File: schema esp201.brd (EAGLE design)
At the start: 100 x 80 mm, 9 parts

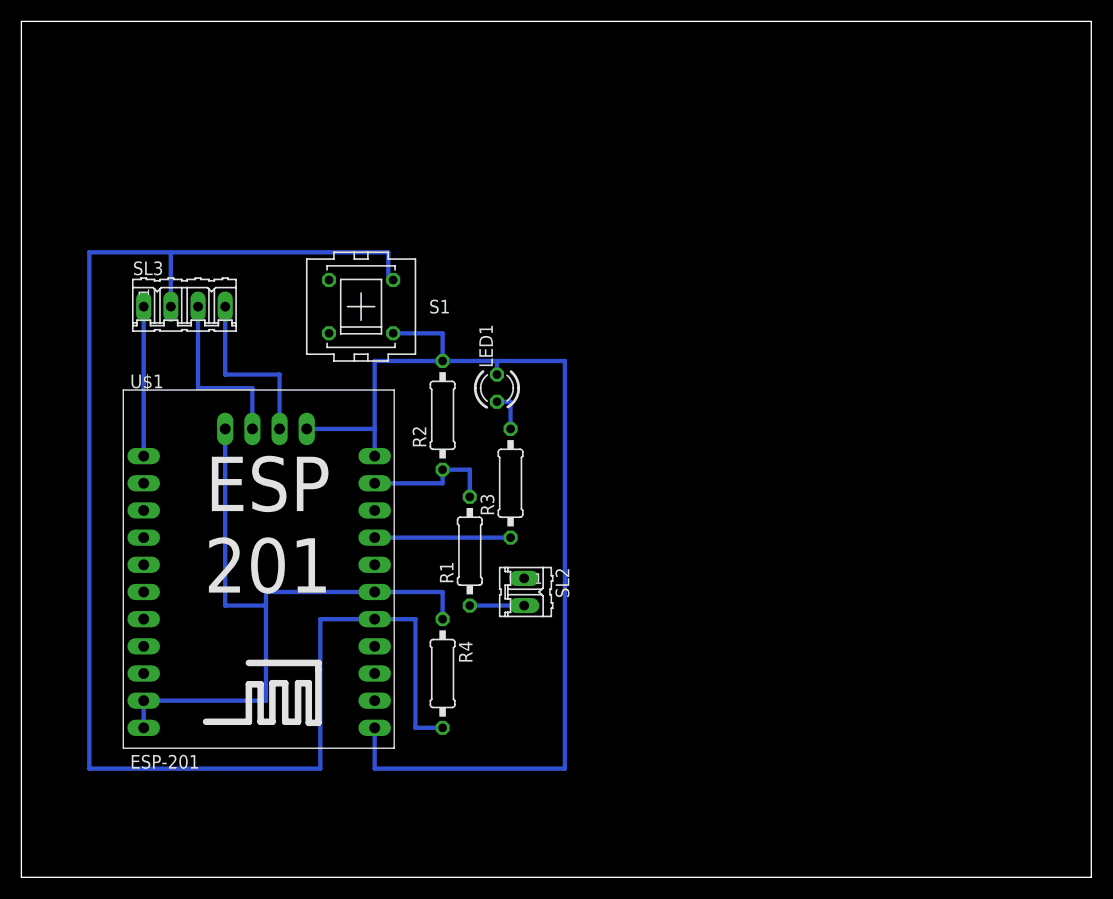
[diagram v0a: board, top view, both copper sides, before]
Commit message: +
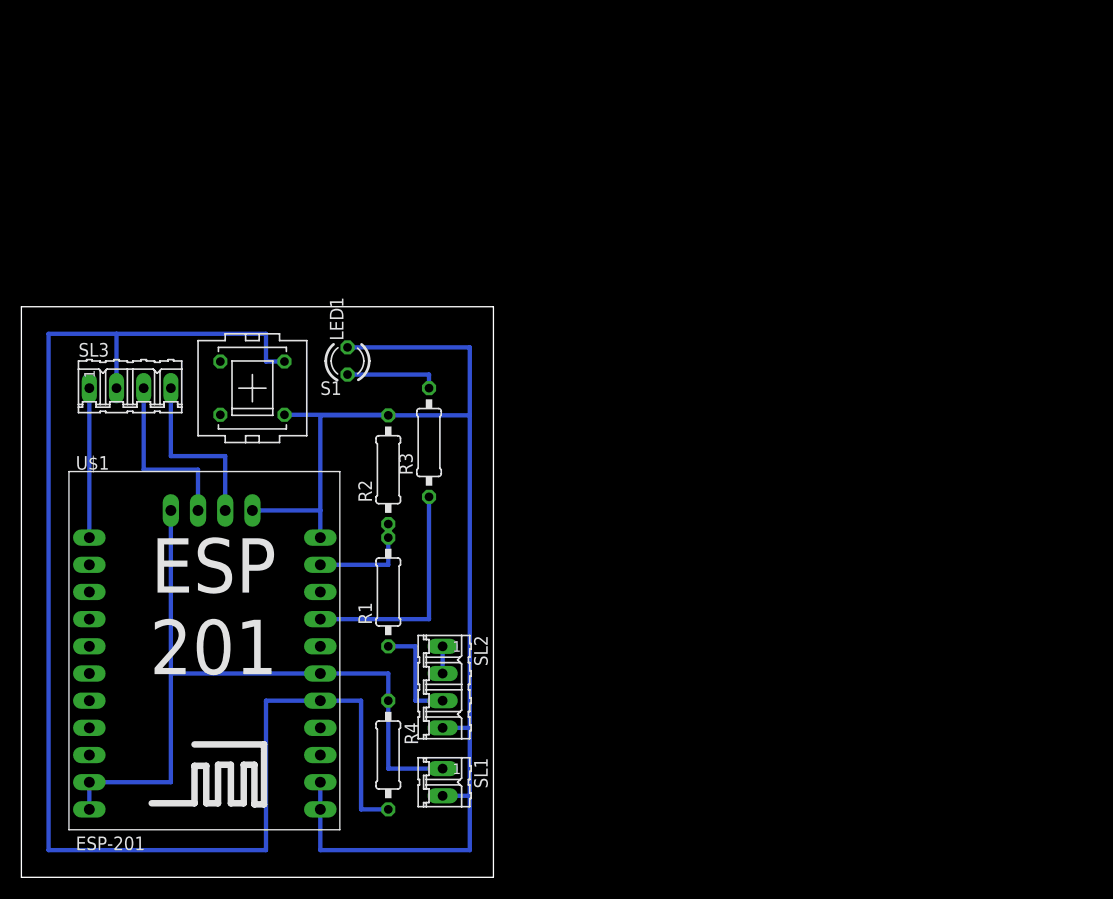
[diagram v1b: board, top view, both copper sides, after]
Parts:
- added SL1: (no value), con-amp-quick:02P
- SL2: device con-amp-quick:02P -> con-amp-quick:04P
- moved LED1 14.2 mm to (30.5, 48.3)
- moved S1 12.7 mm to (21.6, 45.7)
- moved SL2 11.7 mm to (39.4, 17.8)
- moved SL3 9.16 mm to (10.2, 45.7)
- moved U$1 9.16 mm to (6.35, 6.35)
- moved R4 9.16 mm to (34.3, 11.4)
- moved R1 8.52 mm to (34.3, 26.7)
- moved R3 8.52 mm to (38.1, 40.6)
- moved R2 7.18 mm to (34.3, 38.1)
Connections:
- net +12V: now also SL2.2
- net +3V3: now also SL1.1
- net GND: now also SL1.2, SL2.4
- net N$7: now also SL2.3; no longer SL2.2
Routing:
- net GND: track 101.2 -> 125.3 mm
- net N$3: track 12.7 -> 21.6 mm
- net N$4: track 141.5 -> 133.9 mm
- net +3V3: track 63.5 -> 69.8 mm
- net N$1: track 3.81 -> 8.89 mm
- net N$7: track 5.08 -> 10.2 mm
- net +12V: track 0.00 -> 2.54 mm
- net N$2: track 12.7 -> 10.2 mm
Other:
- board size 100 x 80 mm -> 44.1 x 53.3 mm
